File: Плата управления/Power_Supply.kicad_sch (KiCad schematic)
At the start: 21 parts, among them U10 LMV321, U11 LM2594HVM-12, U9 LM2594HVM-12

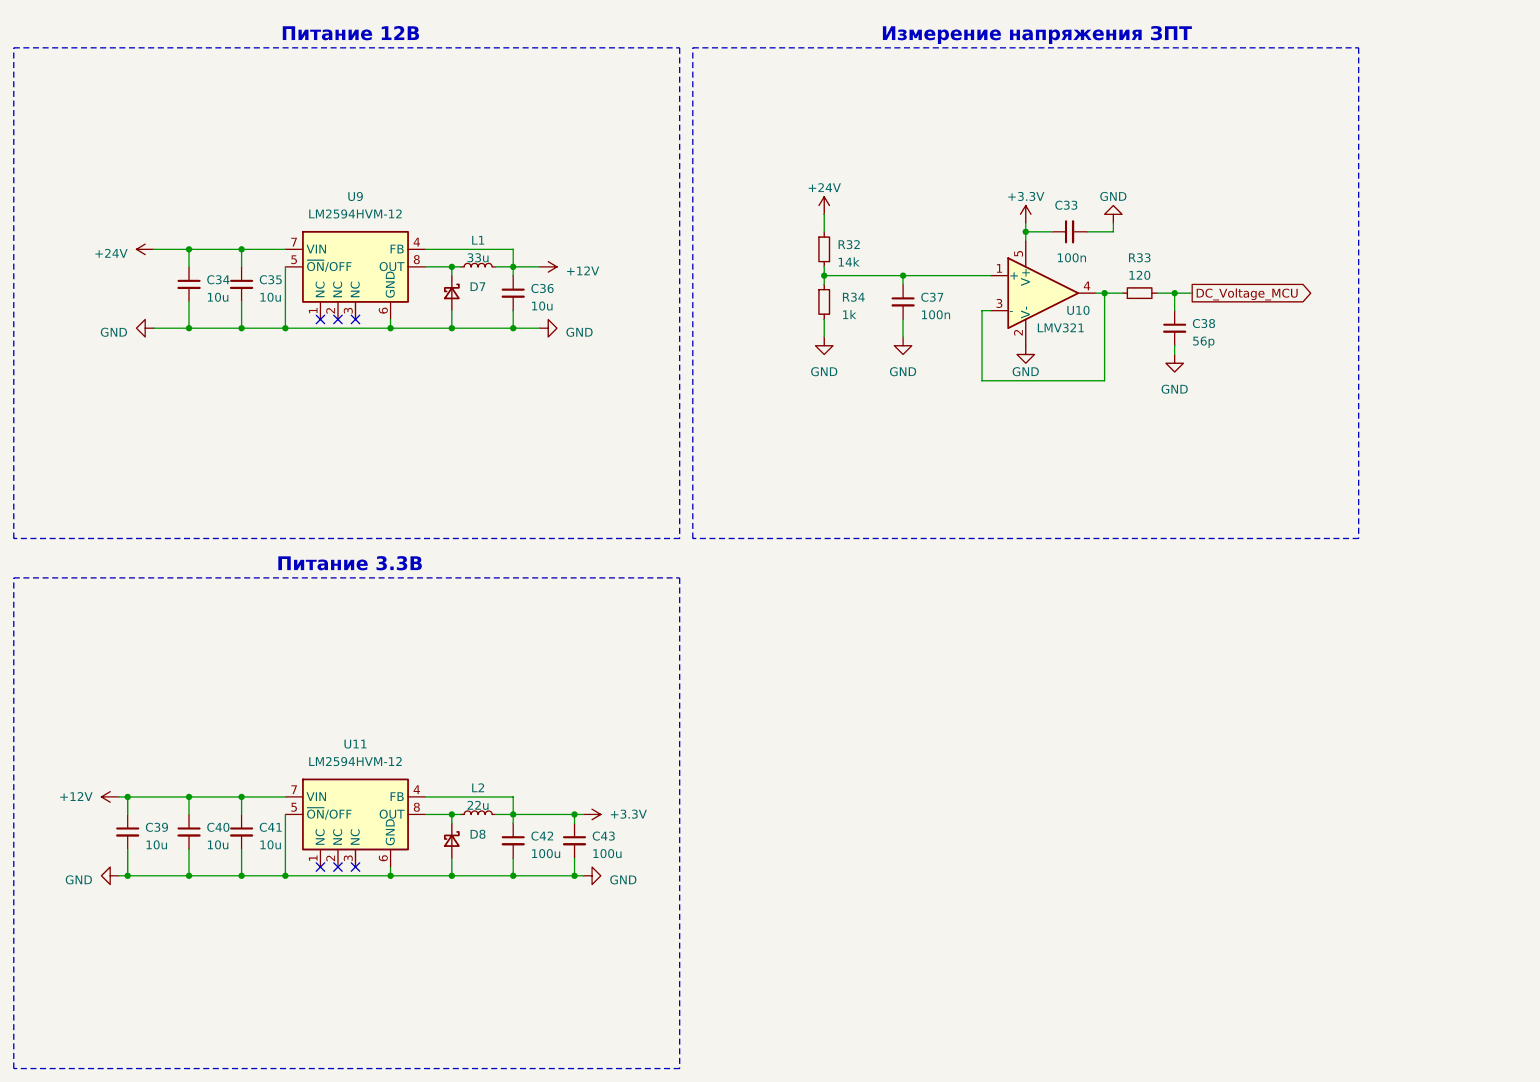
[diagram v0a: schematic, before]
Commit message: Версия под отчёт
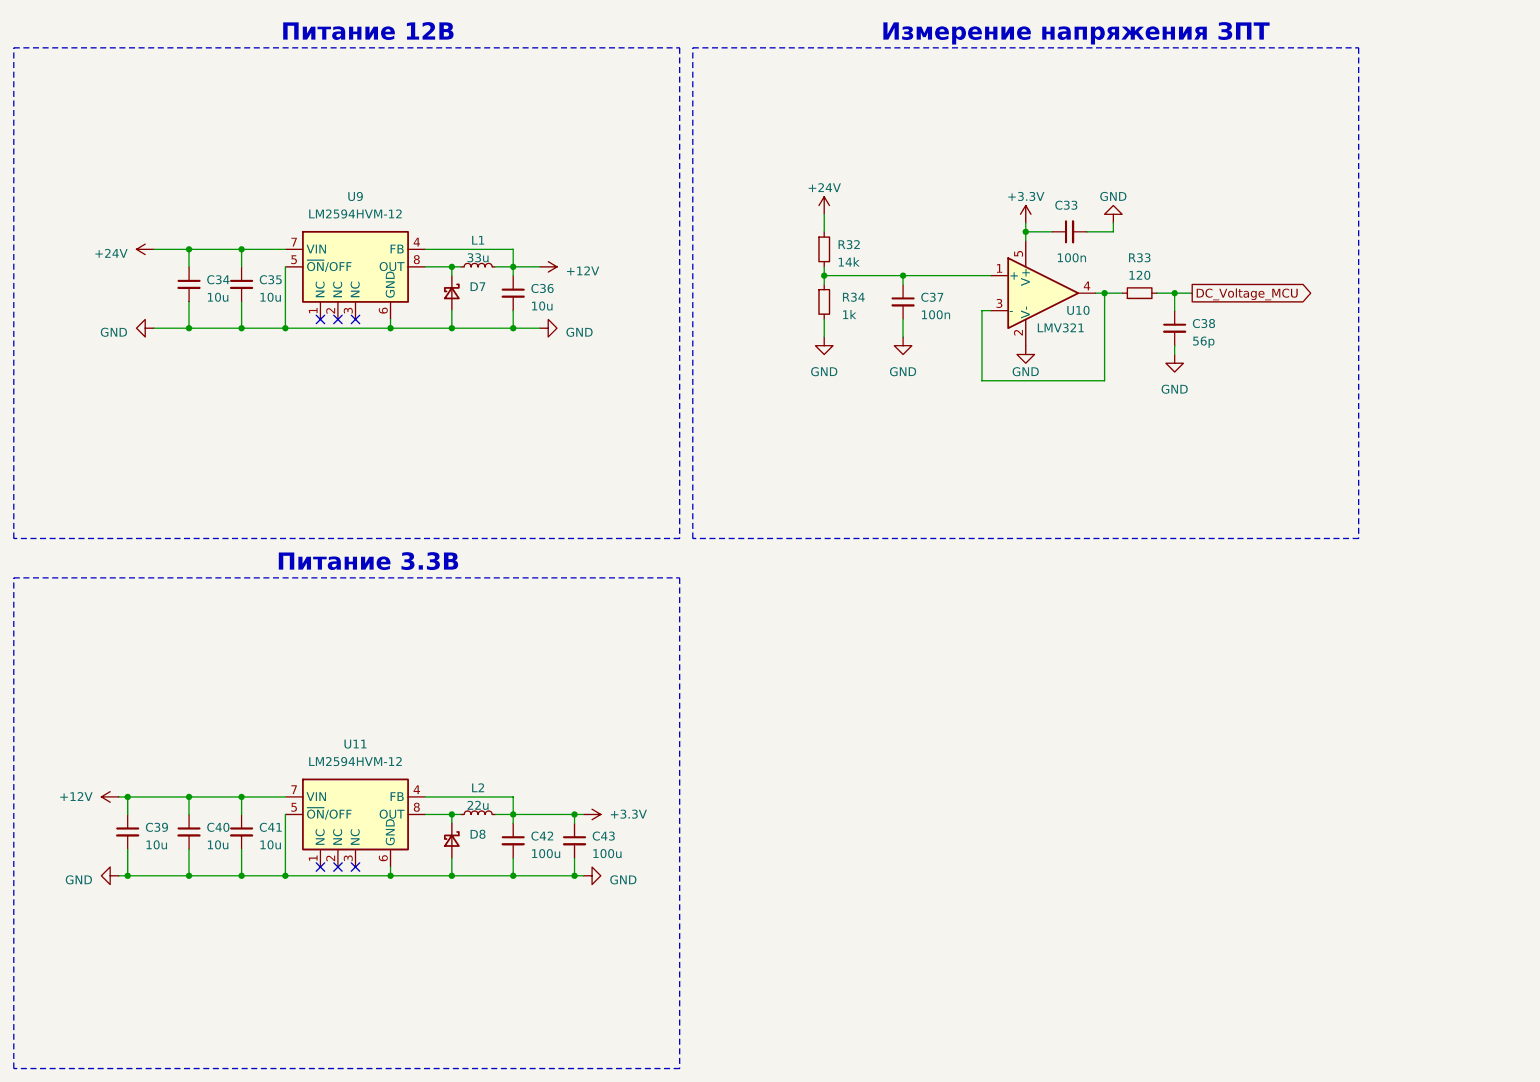
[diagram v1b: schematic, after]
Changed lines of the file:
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@@
   )
   (text "Питание 3.3В" (at 97.79 111.125 0)
-    (effects (font (size 2 2) (thickness 0.4) bold) (justify left bottom))
+    (effects (font (size 2.5 2.5) (thickness 0.4) bold) (justify left bottom))
   )
   (text "Измерение напряжения ЗПТ" (at 185.42 34.29 0)
-    (effects (font (size 2 2) (thickness 0.4) bold) (justify left bottom))
+    (effects (font (size 2.5 2.5) (thickness 0.4) bold) (justify left bottom))
   )
   (text "Питание 12В" (at 98.425 34.29 0)
-    (effects (font (size 2 2) (thickness 0.4) bold) (justify left bottom))
+    (effects (font (size 2.5 2.5) (thickness 0.4) bold) (justify left bottom))
   )
   (global_label "DC_Voltage_MCU" (shape output) (at 230.505 70.485 0) (fields_autoplaced)
